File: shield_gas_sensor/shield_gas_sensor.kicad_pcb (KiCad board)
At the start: 2 copper layers, 132.1 x 63.5 mm, 21 parts, among them P1 Power, P2 Analog, P3 Digital, P4 Digital, P5 CONN_01X01, P6 CONN_01X01, P7 CONN_01X01, P8 CONN_01X01, U1 LTC1050, U2 RN2483_Breakout

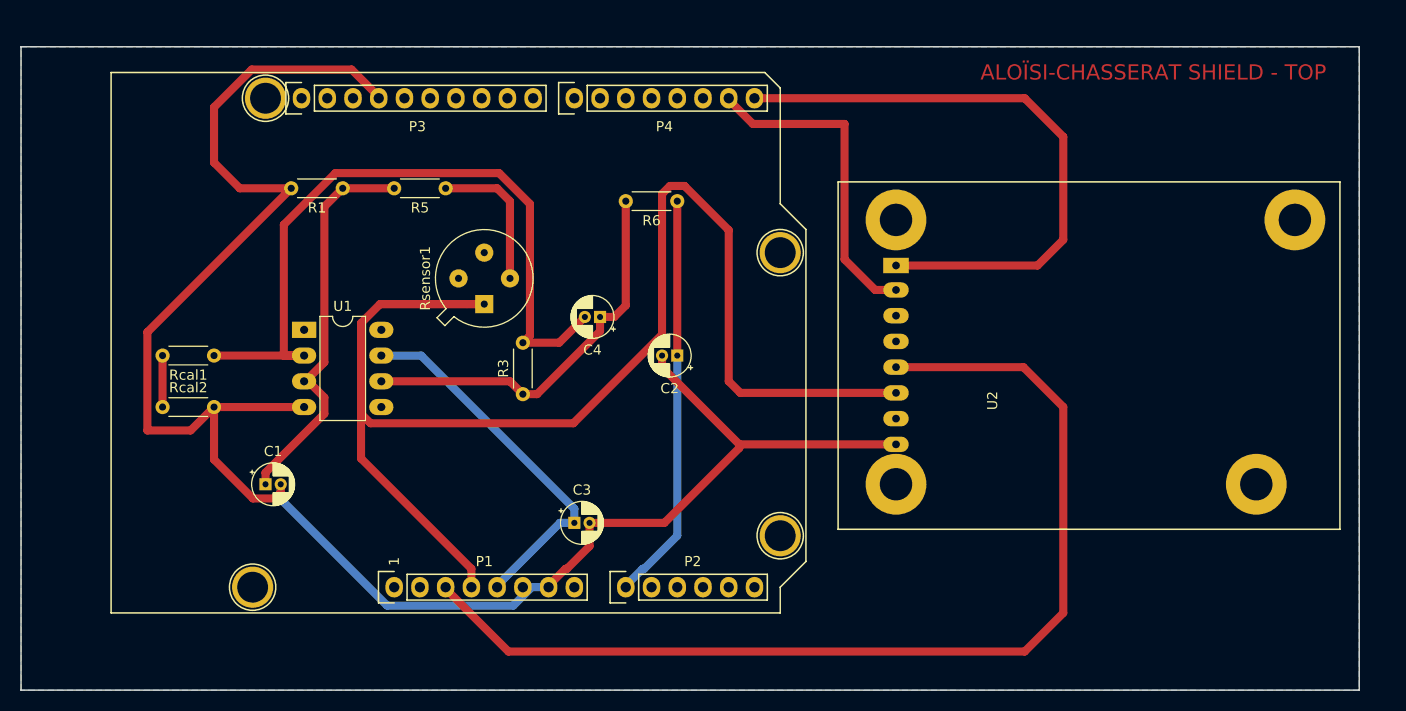
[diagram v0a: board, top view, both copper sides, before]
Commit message: PCB Improvements for realisation at INSA
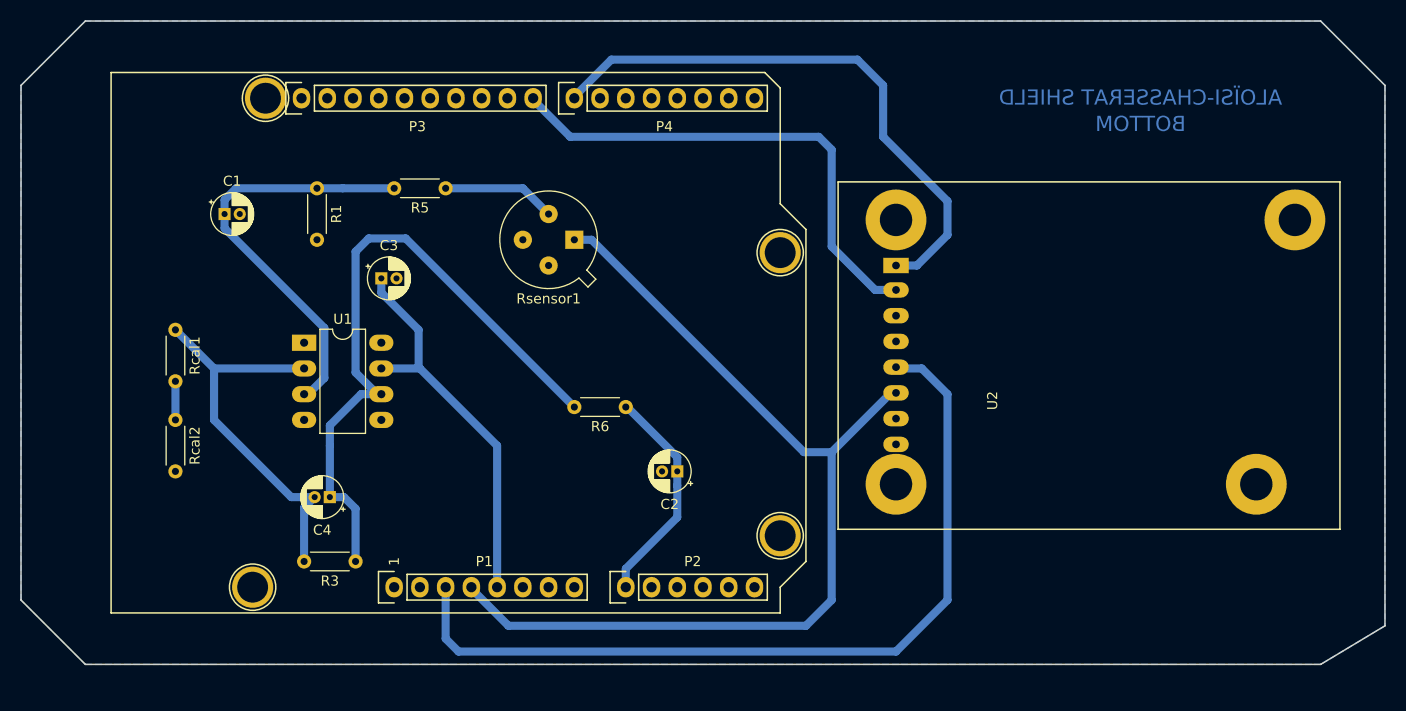
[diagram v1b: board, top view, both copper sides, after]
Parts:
- moved C4 32.1 mm to (132.6, 114.9)
- moved C3 30.7 mm to (137.7, 93.3)
- moved C1 27.0 mm to (122.2, 87.0)
- moved R3 23.3 mm to (135.1, 121.3), turned to 180 degrees
- moved R6 20.9 mm to (161.8, 106.0)
- moved C2 11.4 mm to (166.9, 112.4)
- moved Rsensor1 10.9 mm to (156.7, 89.5), turned to 180 degrees
- moved Rcal1 4.58 mm to (117.3, 98.4), turned to 270 degrees
- moved R1 2.54 mm to (131.3, 84.5), turned to 270 degrees
- moved Rcal2 1.80 mm to (117.3, 107.3), turned to 270 degrees
- moved U1 1.27 mm to (130.0, 99.7)
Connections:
- U2 pad 1: /Rx -> /7
- U2 pad 2: /Tx -> /8
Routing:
- net GND: track 180.5 -> 0.30 mm
- net /Rx: track 59.8 -> 0.00 mm
- net /7: track 0.00 -> 57.1 mm
- net +3V3: track 151.0 -> 95.7 mm
- net /8: track 0.00 -> 49.5 mm
- net Net-(C4-Pad2): track 72.6 -> 39.2 mm
- net /Tx: track 32.3 -> 0.15 mm
- net Net-(C4-Pad1): track 39.4 -> 66.0 mm
- net /Reset: track 103.7 -> 83.9 mm
- net /A0: track 40.3 -> 22.2 mm
- net Net-(R5-Pad1): track 14.5 -> 11.2 mm
- net +5V: track 37.0 -> 39.6 mm
- net Net-(C1-Pad1): track 39.4 -> 41.5 mm
- net Net-(Rcal1-Pad2): track 5.08 -> 3.81 mm
- added copper zone on B.Cu, net GND
- removed copper zone on B.Cu, net (none)
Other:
- board size 132.1 x 63.5 mm -> 134.6 x 63.5 mm
- board text added: "ALOÏSI-CHASSERAT SHIELD"
- board text added: "BOTTOM"
- board text removed: "ALOÏSI-CHASSERAT SHIELD - TOP"
